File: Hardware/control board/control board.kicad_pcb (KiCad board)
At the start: 2 copper layers, 53.3 x 99.1 mm, 33 parts, among them J1 Screw_Terminal_01x02, J10 Screw_Terminal_01x02, J11 Screw_Terminal_01x02, J9 Screw_Terminal_01x02, Q1 NMOS, Q2 NMOS, Q3 NMOS, SW1 SW_Push

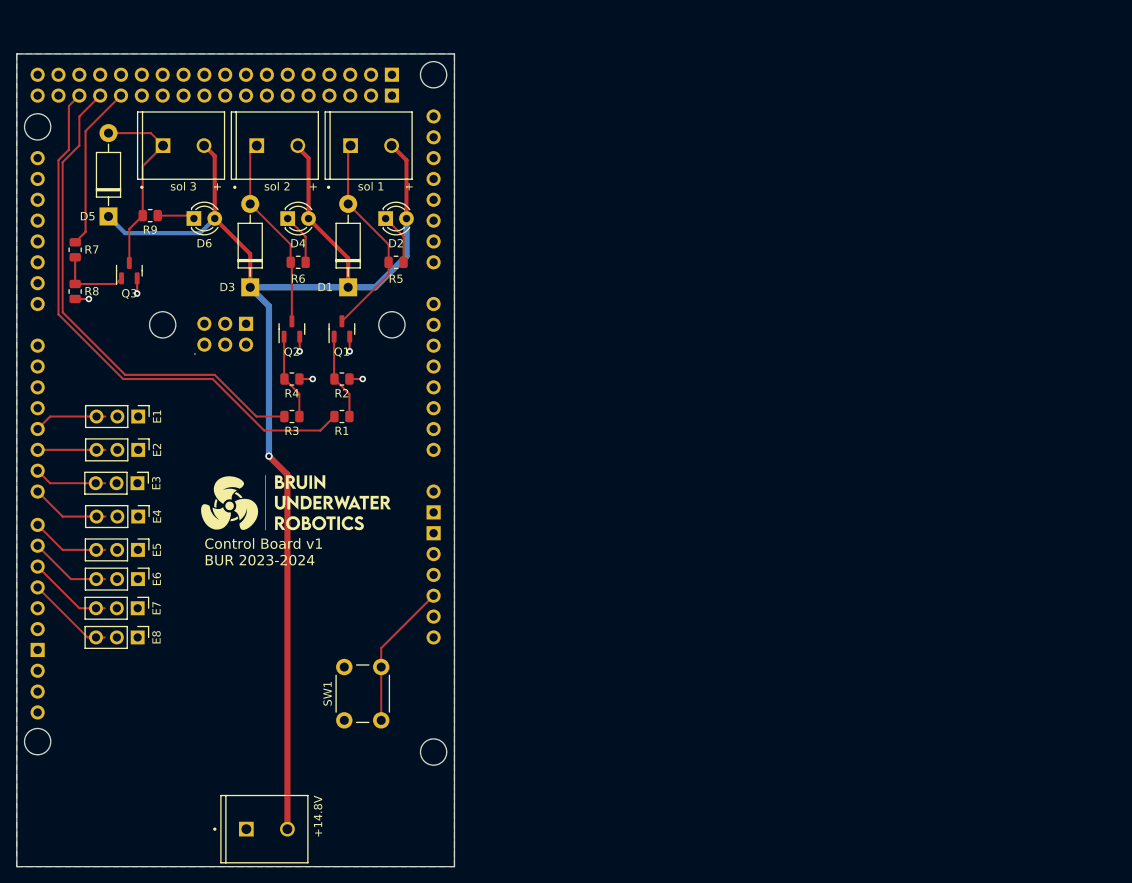
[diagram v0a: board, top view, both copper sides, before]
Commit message: updated Board design to v2
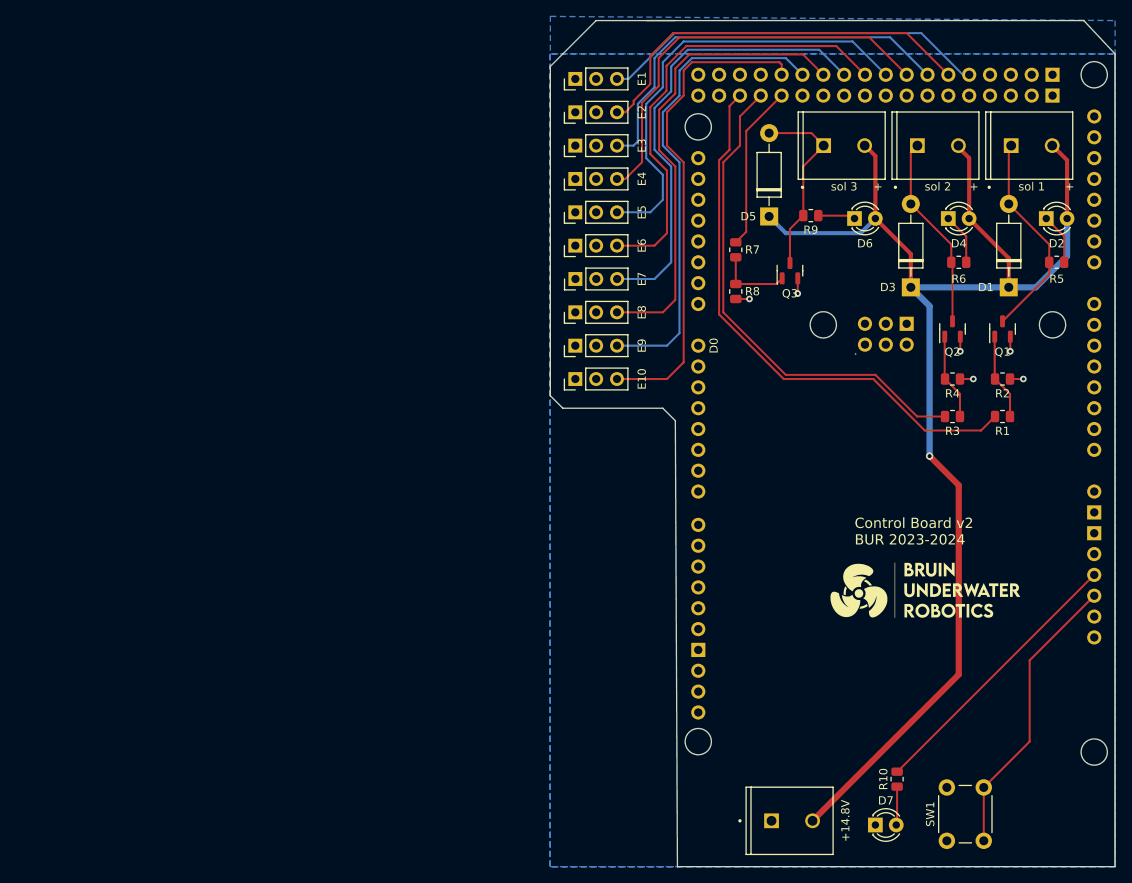
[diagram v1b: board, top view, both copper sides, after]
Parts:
- added D7: LED, LED_THT:LED_D3.0mm_Clear, F.Cu at (136.7, 137.2)
- added E10: Conn_01x03_Pin, Connector_PinHeader_2.54mm:PinHeader_1x03_P2.54mm_Vertical, F.Cu at (100.1, 82.8)
- added E9: Conn_01x03_Pin, Connector_PinHeader_2.54mm:PinHeader_1x03_P2.54mm_Vertical, F.Cu at (100.1, 78.7)
- added R10: 100, Resistor_SMD:R_0805_2012Metric, F.Cu at (139.3, 131.6)
- A1: footprint PCM_arduino-library:Arduino_Mega2560_R3_Shield -> PCM_arduino-library:Arduino_Due_Shield
- moved J11 80.5 mm to (132.8, 54.4)
- moved Q2 80.5 mm to (146.1, 76.7)
- moved R3 80.5 mm to (146.1, 87.4)
- moved R4 80.5 mm to (146.1, 82.8)
- moved R6 80.5 mm to (146.8, 68.6)
- moved A1 80.5 mm to (165.9, 142.2)
- moved D2 80.5 mm to (157.5, 63.2)
- moved D3 80.5 mm to (141.0, 71.6)
- moved D4 80.5 mm to (145.5, 63.2)
- moved D5 80.5 mm to (123.7, 63.0)
- moved D6 80.5 mm to (134.1, 63.2)
- moved J10 80.5 mm to (144.3, 54.4)
- moved J9 80.5 mm to (155.7, 54.4)
- moved Q3 80.5 mm to (126.2, 69.6)
- moved R5 80.5 mm to (158.8, 68.6)
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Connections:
- A1 pad 3V3: unconnected-(A1-3.3V-Pad3V3) -> Net-(A1-3.3V)
- A1 pad D10: /PWMD10 -> unconnected-(A1-D10_CS0-PadD10)
- A1 pad D11: /PWMD11 -> unconnected-(A1-PadD11)
- A1 pad D29: unconnected-(A1-PadD29) -> Net-(E10-Pin_3)
- A1 pad D31: unconnected-(A1-PadD31) -> Net-(E9-Pin_3)
- A1 pad D33: unconnected-(A1-PadD33) -> Net-(E8-Pin_3)
- A1 pad D35: unconnected-(A1-PadD35) -> Net-(E7-Pin_3)
- A1 pad D37: unconnected-(A1-PadD37) -> Net-(E6-Pin_3)
- A1 pad D39: unconnected-(A1-PadD39) -> Net-(E5-Pin_3)
- A1 pad D4: /PWMD4 -> unconnected-(A1-D4_CS1-PadD4)
- A1 pad D41: unconnected-(A1-PadD41) -> Net-(E4-Pin_3)
- A1 pad D43: unconnected-(A1-PadD43) -> Net-(E3-Pin_3)
- A1 pad D45: unconnected-(A1-PadD45) -> Net-(E2-Pin_3)
- A1 pad D47: unconnected-(A1-PadD47) -> Net-(E1-Pin_3)
- A1 pad D5: /PWMD5 -> unconnected-(A1-PadD5)
- A1 pad D6: /PWMD6 -> unconnected-(A1-PadD6)
- A1 pad D7: /PWMD7 -> unconnected-(A1-PadD7)
- A1 pad D8: /PWMD8 -> unconnected-(A1-PadD8)
- A1 pad D9: /PWMD9 -> unconnected-(A1-PadD9)
- E1 pad 3: /PWMD4 -> Net-(E1-Pin_3)
- E2 pad 3: /PWMD5 -> Net-(E2-Pin_3)
- E3 pad 3: /PWMD6 -> Net-(E3-Pin_3)
- E4 pad 3: /PWMD7 -> Net-(E4-Pin_3)
- E5 pad 3: /PWMD8 -> Net-(E5-Pin_3)
- E6 pad 3: /PWMD9 -> Net-(E6-Pin_3)
- E7 pad 3: /PWMD10 -> Net-(E7-Pin_3)
- E8 pad 3: /PWMD11 -> Net-(E8-Pin_3)
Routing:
- net Net-(E10-Pin_3): track 0.00 -> 59.9 mm
- net Net-(E9-Pin_3): track 0.00 -> 58.4 mm
- net Net-(E8-Pin_3): track 0.00 -> 57.3 mm
- net Net-(E7-Pin_3): track 0.00 -> 56.2 mm
- net Net-(E6-Pin_3): track 0.00 -> 55.4 mm
- net Net-(E5-Pin_3): track 0.00 -> 54.6 mm
- net Net-(E4-Pin_3): track 0.00 -> 50.6 mm
- net Net-(E3-Pin_3): track 0.00 -> 50.0 mm
- net Net-(E2-Pin_3): track 0.00 -> 48.7 mm
- net Net-(E1-Pin_3): track 0.00 -> 47.3 mm
- net Net-(A1-3.3V): track 0.00 -> 34.0 mm
- net Net-(A1-RESET): track 17.1 -> 35.4 mm
- net /PWMD11: track 10.7 -> 0.00 mm
- net /PWMD10: track 10.3 -> 0.00 mm
- net /PWMD9: track 9.91 -> 0.00 mm
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- added copper zone on B.Cu, net (none)
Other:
- board size 53.3 x 99.1 mm -> 68.8 x 103.1 mm
- board text added: "Control Board v2 BUR 2023-2024"
- board text removed: "Control Board v1 BUR 2023-2024"

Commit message: layout cleanup
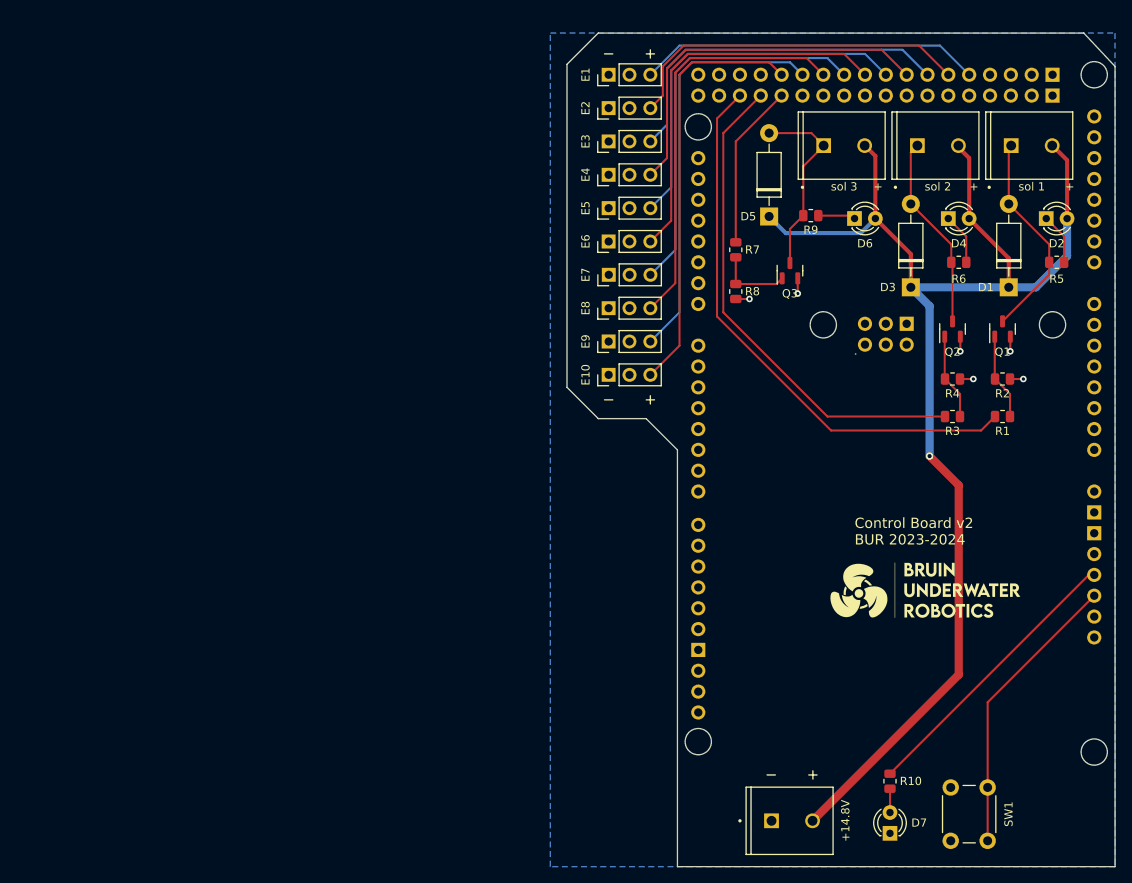
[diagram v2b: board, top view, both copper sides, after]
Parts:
- moved E1 4.10 mm to (104.1, 45.7)
- moved E10 4.10 mm to (104.1, 82.3)
- moved E2 4.10 mm to (104.1, 49.8)
- moved E3 4.10 mm to (104.1, 53.8)
- moved E4 4.10 mm to (104.1, 57.9)
- moved E5 4.10 mm to (104.1, 62.0)
- moved E6 4.10 mm to (104.1, 66.0)
- moved E7 4.10 mm to (104.2, 70.1)
- moved E8 4.10 mm to (104.1, 74.2)
- moved E9 4.10 mm to (104.1, 78.2)
- moved D7 2.05 mm to (138.4, 138.2), turned to 90 degrees
- moved R10 0.90 mm to (138.4, 131.8)
- moved SW1 0.47 mm to (145.8, 139.1)
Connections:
- net Net-(E1-Pin_3) renamed /esc 1
- net Net-(E10-Pin_3) renamed /esc 10
- net Net-(E2-Pin_3) renamed /esc 2
- net Net-(E3-Pin_3) renamed /esc 3
- net Net-(E4-Pin_3) renamed /esc 4
- net Net-(E5-Pin_3) renamed /esc 5
- net Net-(E6-Pin_3) renamed /esc 6
- net Net-(E7-Pin_3) renamed /esc 7
- net Net-(E8-Pin_3) renamed /esc 8
- net Net-(E9-Pin_3) renamed /esc 9
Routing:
- net /esc 5: track 54.6 -> 45.9 mm
- net /esc 10: track 59.9 -> 51.8 mm
- net /esc 9: track 58.4 -> 50.2 mm
- net /esc 7: track 56.2 -> 48.0 mm
- net /esc 6: track 55.4 -> 47.4 mm
- net /esc 8: track 57.3 -> 49.6 mm
- net /esc 3: track 50.0 -> 43.7 mm
- net /esc 2: track 48.7 -> 43.0 mm
- net /esc 1: track 47.3 -> 41.8 mm
- net /esc 4: track 50.6 -> 45.2 mm
- net Net-(D7-A): track 4.72 -> 2.90 mm
- net Net-(A1-3.3V): track 34.0 -> 34.9 mm
- net /sol 1: track 67.9 -> 68.4 mm
- removed copper zone on B.Cu, net (none)
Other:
- board size 68.8 x 103.1 mm -> 66.8 x 101.6 mm
